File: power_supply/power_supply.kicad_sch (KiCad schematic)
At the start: 30 parts, among them J1 Conn_01x02_Socket, J10 Conn_01x02_Socket, J11 Conn_01x02_Socket, J12 Conn_01x02_Socket, J13 Conn_01x02_Socket, J14 Conn_01x02_Socket, J15 Conn_01x02_Socket, J16 Conn_01x02_Socket, J17 Conn_01x02_Socket, J18 Conn_01x02_Socket, J19 Conn_01x02_Socket, J2 Conn_01x02_Socket, J20 Conn_01x02_Socket, J21 Conn_01x02_Pin, J22 Conn_01x02_Pin, J23 Conn_01x02_Socket, J24 Conn_01x02_Socket, J3 Conn_01x02_Socket, J4 Conn_01x02_Socket, J5 Conn_01x02_Socket, J6 Conn_01x02_Socket, J7 Conn_01x02_Socket, J8 Conn_01x02_Socket, J9 Conn_01x02_Socket

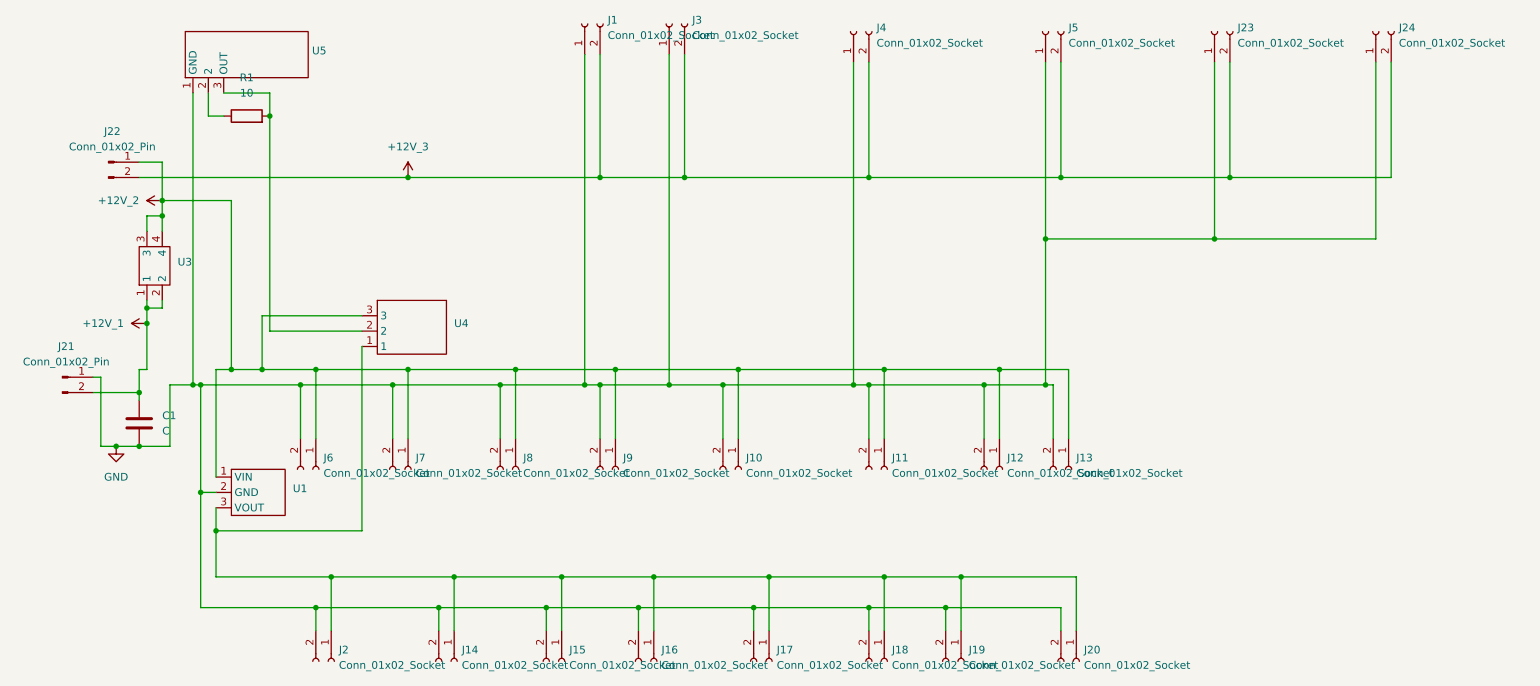
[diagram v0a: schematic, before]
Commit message: 2024/11/05/23:24
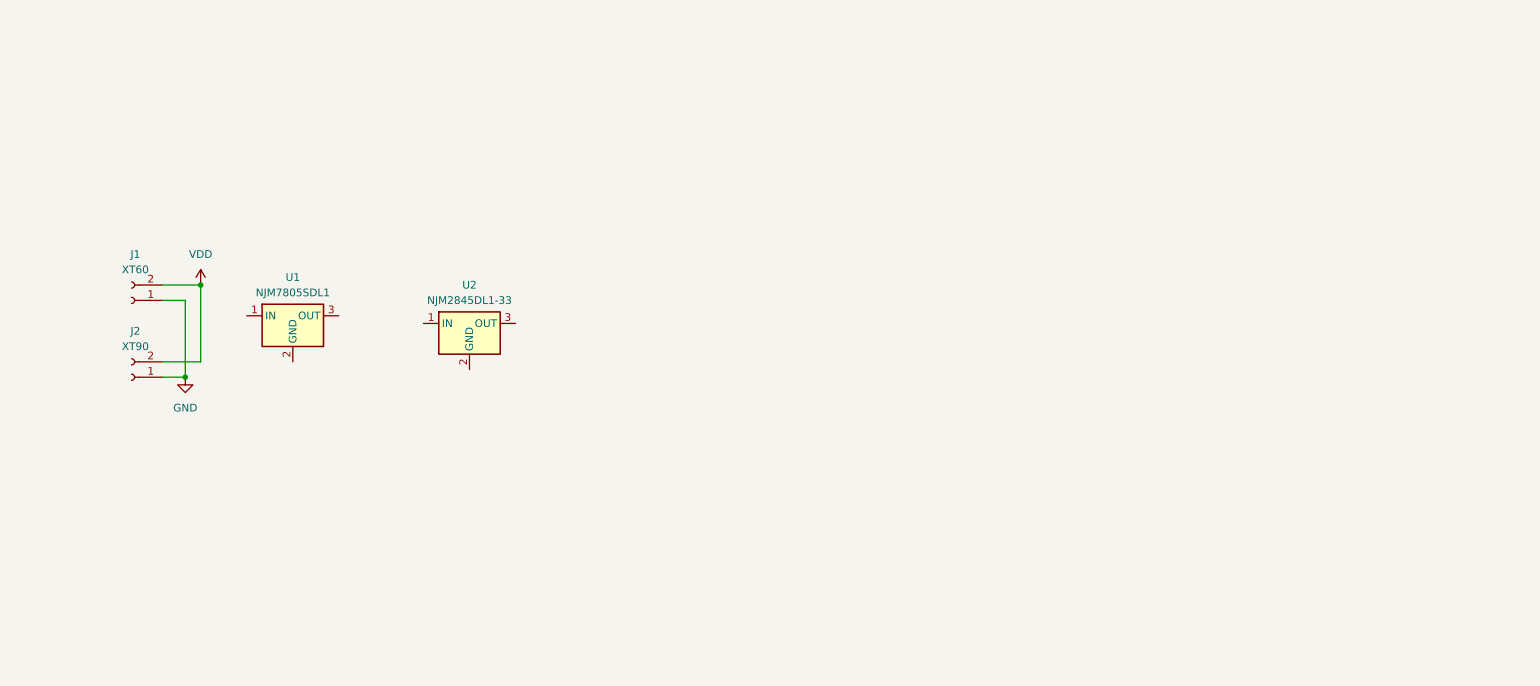
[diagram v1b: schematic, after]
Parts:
- removed C1: C, Connector_PinHeader_2.54mm:PinHeader_2x01_P2.54mm_Vertical, symbol Device:C
- removed J10, J11, J12, J13, J14, J15, J16, J17, J18, J19, J20, J6, J7, J8, J9: Conn_01x02_Socket, Connector_JST:JST_XH_B2B-XH-A_1x02_P2.50mm_Vertical, symbol Connector:Conn_01x02_Socket
- removed J21, J22: Conn_01x02_Pin, Connector_AMASS:AMASS_XT60-F_1x02_P7.20mm_Vertical, symbol Connector:Conn_01x02_Pin
- removed J23, J24, J3, J4, J5: Conn_01x02_Socket, Connector_AMASS:AMASS_XT60-F_1x02_P7.20mm_Vertical, symbol Connector:Conn_01x02_Socket
- removed R1: 10, Resistor_THT:R_Axial_DIN0207_L6.3mm_D2.5mm_P10.16mm_Horizontal, symbol Device:R
- removed U1: ~, Connector_PinSocket_2.54mm:PinSocket_1x03_P2.54mm_Vertical, symbol 00_a:LXDC55
- removed U3: ~, footprints:3557-15_KEY, symbol 00_a:fuse
- removed U4: ~, 00a:1MS1-T1-B1-M1-Q-N-S, symbol 00_a:Switch(1MS1-T1-B1-M1-Q-N)
- removed U5: ~, Connector_PinHeader_2.54mm:PinHeader_1x03_P2.54mm_Vertical, symbol 00_a:voltmeter-Red(4530)
- added U1: NJM7805SDL1, Converter_DCDC:Converter_DCDC_NJM7805FA, symbol 00a:3pin_regulator
- added U2: NJM2845DL1-33, Converter_DCDC:Converter_DCDC_NJM7805FA, symbol 00a:3pin_regulator
- J1: value Conn_01x02_Socket -> XT60; footprint Connector_AMASS:AMASS_XT60-F_1x02_P7.20mm_Vertical -> (none)
- J2: value Conn_01x02_Socket -> XT90; footprint Connector_JST:JST_XH_B2B-XH-A_1x02_P2.50mm_Vertical -> (none)
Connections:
- net GND: now also J2.1 (Pin_1); no longer J2.2 (Pin_2)
- net +12V_3 renamed VDD
- net VDD: now also J2.2 (Pin_2)
